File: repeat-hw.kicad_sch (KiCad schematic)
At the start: 0 parts

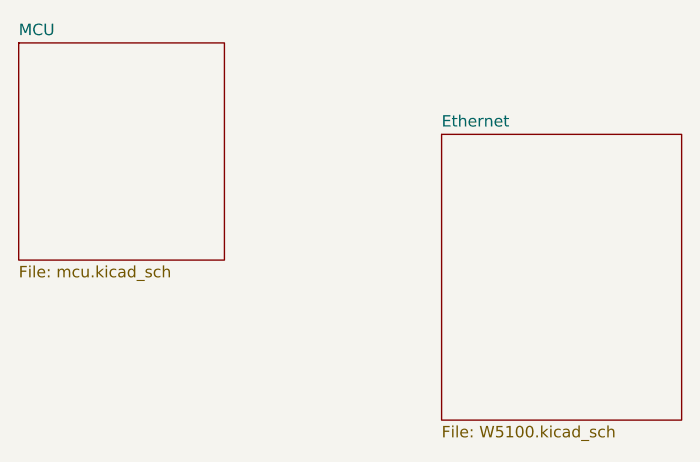
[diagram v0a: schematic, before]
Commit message: Finishe PoE and ethernet
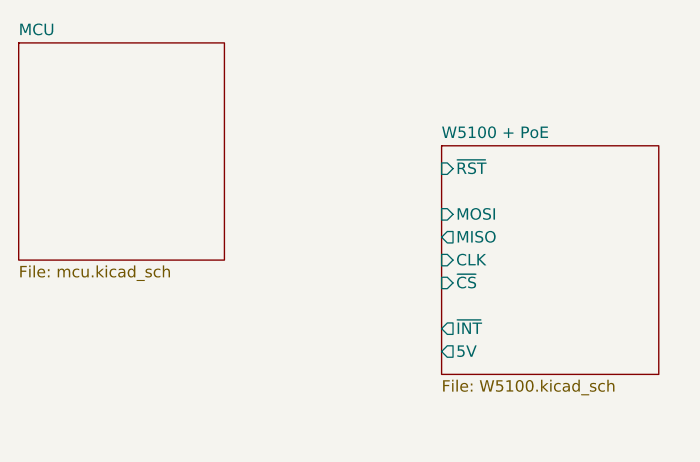
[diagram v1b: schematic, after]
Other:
- sheet Ethernet renamed W5100 + PoE
- sheet W5100 + PoE ports: added 5V, CLK, MISO, MOSI, ~{CS}, ~{INT}, ~{RST}; removed none
